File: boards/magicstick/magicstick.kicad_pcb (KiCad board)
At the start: 2 copper layers, 77.5 x 30.5 mm, 22 parts, among them Q1 2N2222, Q2 2N2222, Q3 2N2222, Q4 2N2907, Q5 2N2907, Q6 2N2907, U1 NodeMCU_Amica_R2

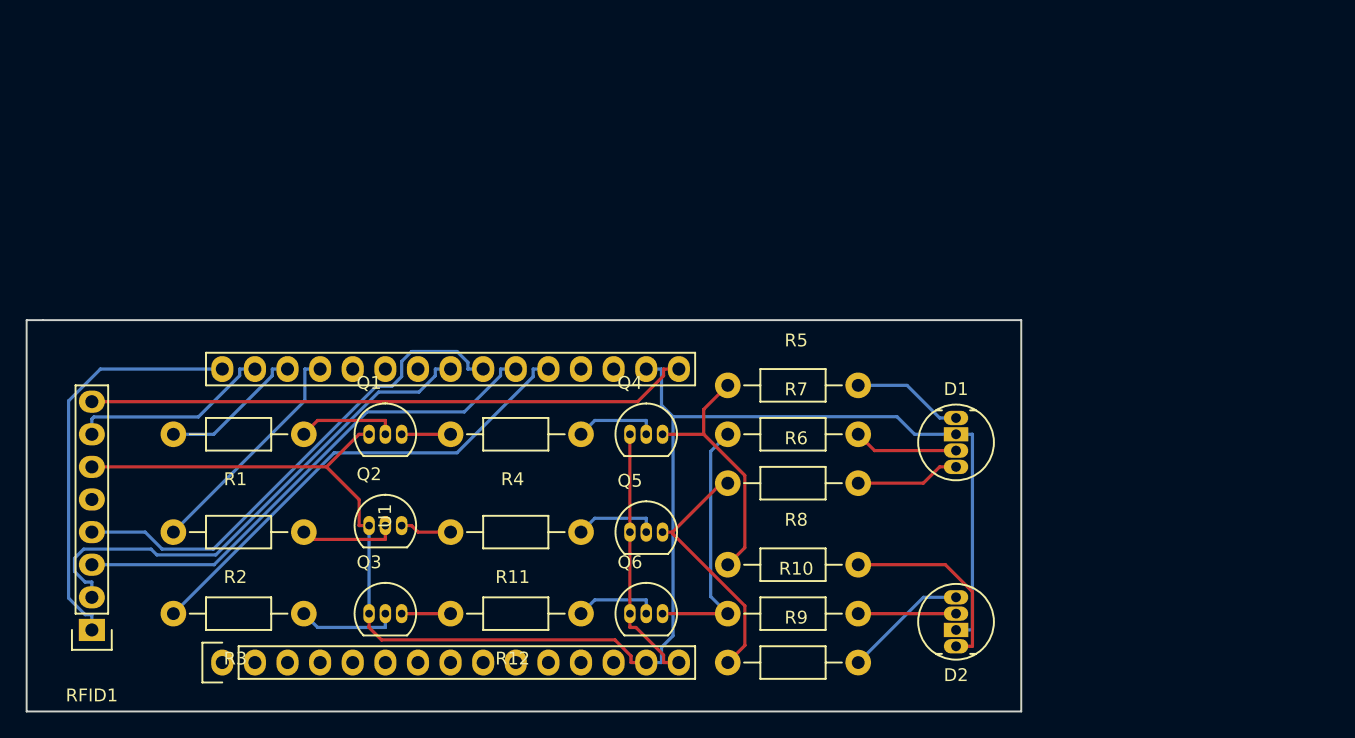
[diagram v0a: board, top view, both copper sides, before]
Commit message: magic stick updates
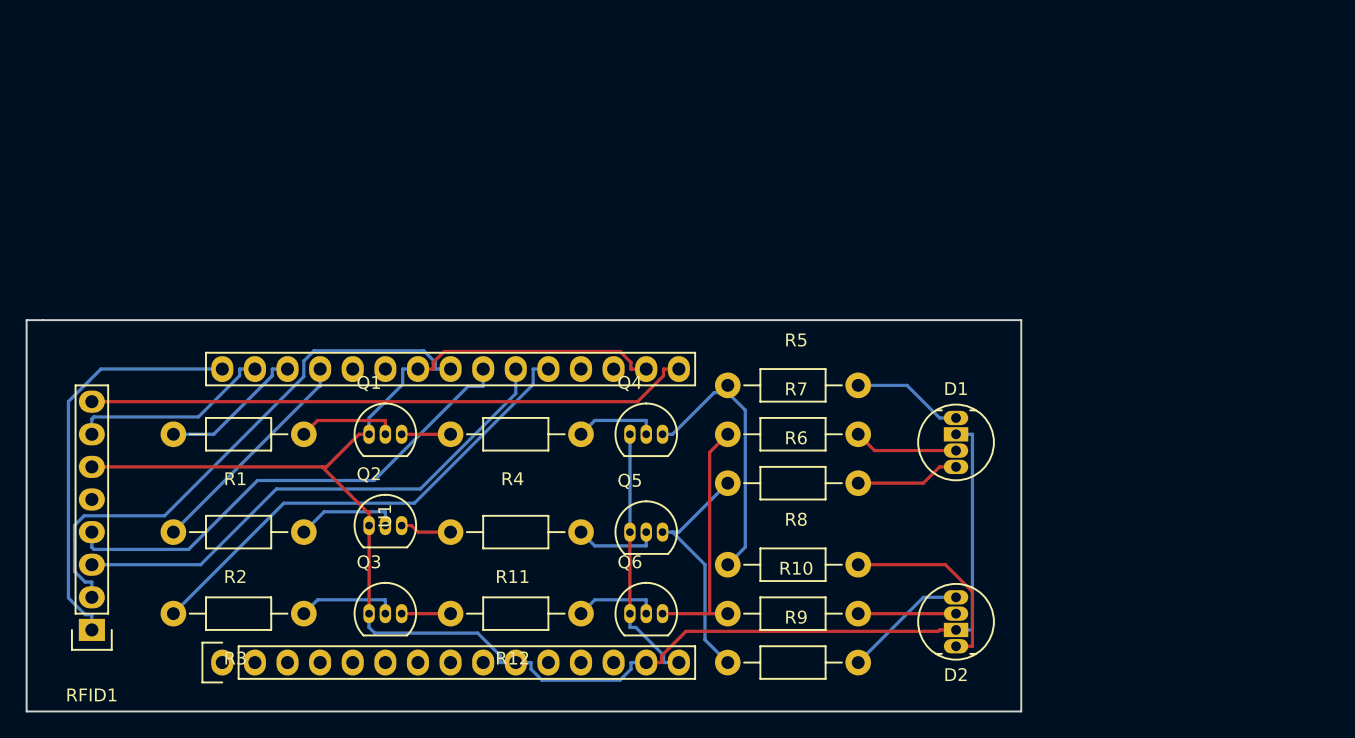
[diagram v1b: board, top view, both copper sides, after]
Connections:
- U1 pad 10: Net-(U1-Pad10) -> GND
- U1 pad 24: Net-(U1-Pad24) -> GND
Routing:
- net GND: track 126.4 -> 131.7 mm
- net Net-(RFID1-Pad2): track 40.0 -> 43.0 mm
- net Net-(Q4-Pad3): track 19.8 -> 21.5 mm
- net Net-(Q5-Pad3): track 19.7 -> 18.6 mm
- net Net-(RFID1-Pad3): track 39.6 -> 40.5 mm
- net Net-(R2-Pad2): track 18.1 -> 17.5 mm
- net Net-(RFID1-Pad4): track 39.0 -> 38.3 mm
- net Net-(Q6-Pad3): track 20.2 -> 19.6 mm

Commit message: initial mother board
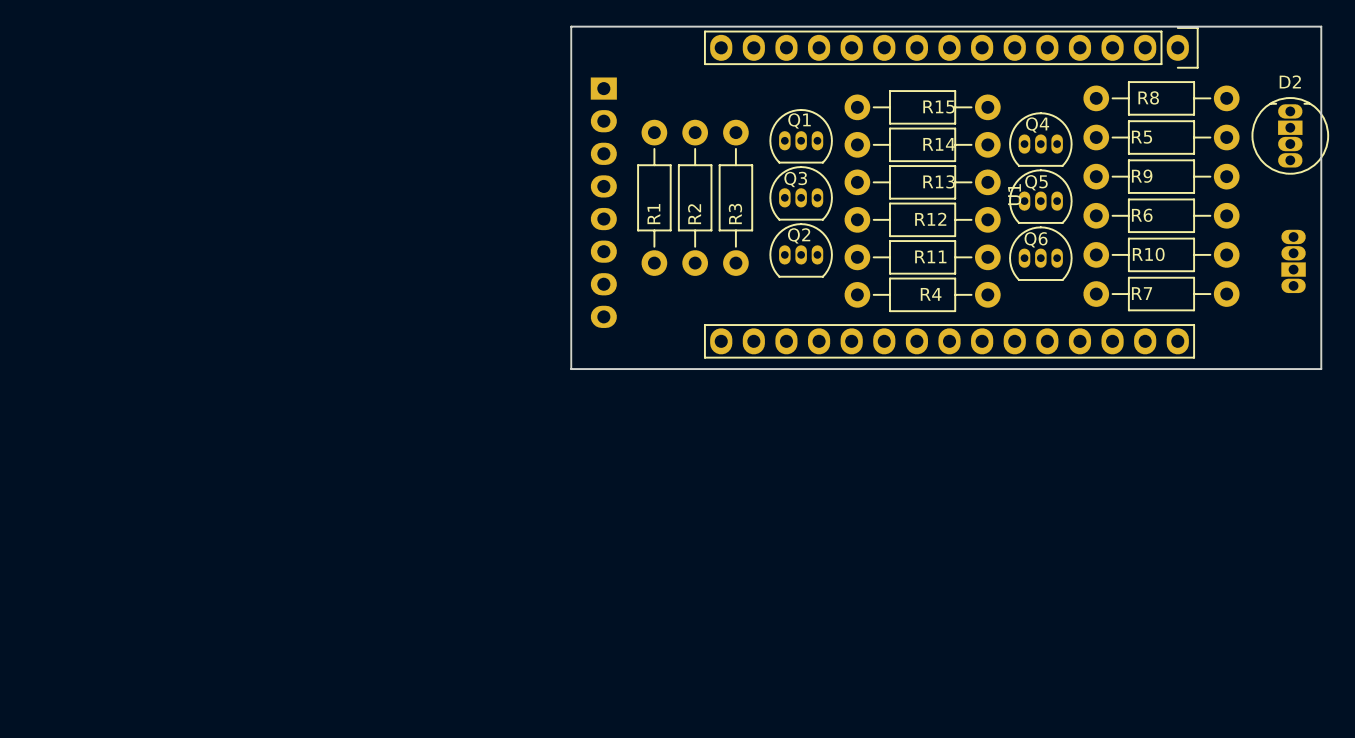
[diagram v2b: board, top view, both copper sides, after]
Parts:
- added R13: 10k, Resistors_ThroughHole:Resistor_Horizontal_RM10mm, F.Cu at (177.7, 50.2)
- added R14: 10k, Resistors_ThroughHole:Resistor_Horizontal_RM10mm, F.Cu at (177.7, 47.3)
- added R15: 10k, Resistors_ThroughHole:Resistor_Horizontal_RM10mm, F.Cu at (177.7, 44.4)
- D1, RFID1: moved to B.Cu
- moved U1 88.5 mm to (192.5, 39.8), turned to 270 degrees
- moved RFID1 58.0 mm to (147.8, 42.9)
- moved D2 49.1 mm to (201.3, 44.7), turned to 0 degrees
- moved R9 47.5 mm to (186.2, 49.8)
- moved R8 46.3 mm to (186.2, 43.7)
- moved Q3 45.8 mm to (161.9, 51.4)
- moved R12 44.1 mm to (177.7, 53.1)
- moved R3 43.3 mm to (158.1, 56.5), turned to 90 degrees
- moved Q6 41.4 mm to (180.6, 56.1)
- moved Q5 40.1 mm to (180.6, 51.7)
- moved R10 40.1 mm to (186.2, 55.9)
- moved Q1 39.6 mm to (161.9, 47.0)
- moved Q2 38.6 mm to (161.9, 55.9)
- moved R11 38.2 mm to (177.7, 56.1)
- moved Q4 38.2 mm to (180.6, 47.2)
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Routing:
- net GND: track 131.7 -> 0.00 mm
- net Net-(RFID1-Pad8): track 47.1 -> 0.00 mm
- net Net-(RFID1-Pad2): track 43.0 -> 0.00 mm
- net Net-(RFID1-Pad3): track 40.5 -> 0.00 mm
- net Net-(RFID1-Pad4): track 38.3 -> 0.00 mm
- net Net-(R3-Pad2): track 37.8 -> 0.00 mm
- net Net-(RFID1-Pad1): track 31.9 -> 0.00 mm
- net Net-(Q4-Pad3): track 21.5 -> 0.00 mm
- net +5V: track 20.3 -> 0.00 mm
- net Net-(Q6-Pad3): track 19.6 -> 0.00 mm
- net Net-(Q5-Pad3): track 18.6 -> 0.00 mm
- net Net-(R2-Pad2): track 17.5 -> 0.00 mm
- net Net-(RFID1-Pad7): track 15.8 -> 0.00 mm
- net Net-(D2-Pad1): track 15.3 -> 0.00 mm
- net Net-(R1-Pad2): track 11.3 -> 0.00 mm
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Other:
- board size 77.5 x 30.5 mm -> 58.4 x 26.7 mm
- net class Power added: clearance 0.2, trace_width 0.5, via_dia 0.6, via_drill 0.4
